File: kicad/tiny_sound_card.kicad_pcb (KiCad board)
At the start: 2 copper layers, 91 x 55 mm, 46 parts, among them CON1 BARREL_JACK, IC1 ATMEGA328P-A, J1 TRS_JACK, M1 DFR0299, P1 EXT_PWR, P10 M3Drill, P2 SPKOUT, P4 EXT_I2C, P4 M3Drill, P5 EXT_SW0, P6 EXT_UART, P7 EXT_SPI/ISP, P8 M3Drill, P9 M3Drill, SW1 SlideSW, SW2 SW_PUSH, SW3 SW_PUSH, SW4 SW_PUSH, SW5 SlideSW, SW6 SW_PUSH, U1 STMPS2141S, Y1 16MHz

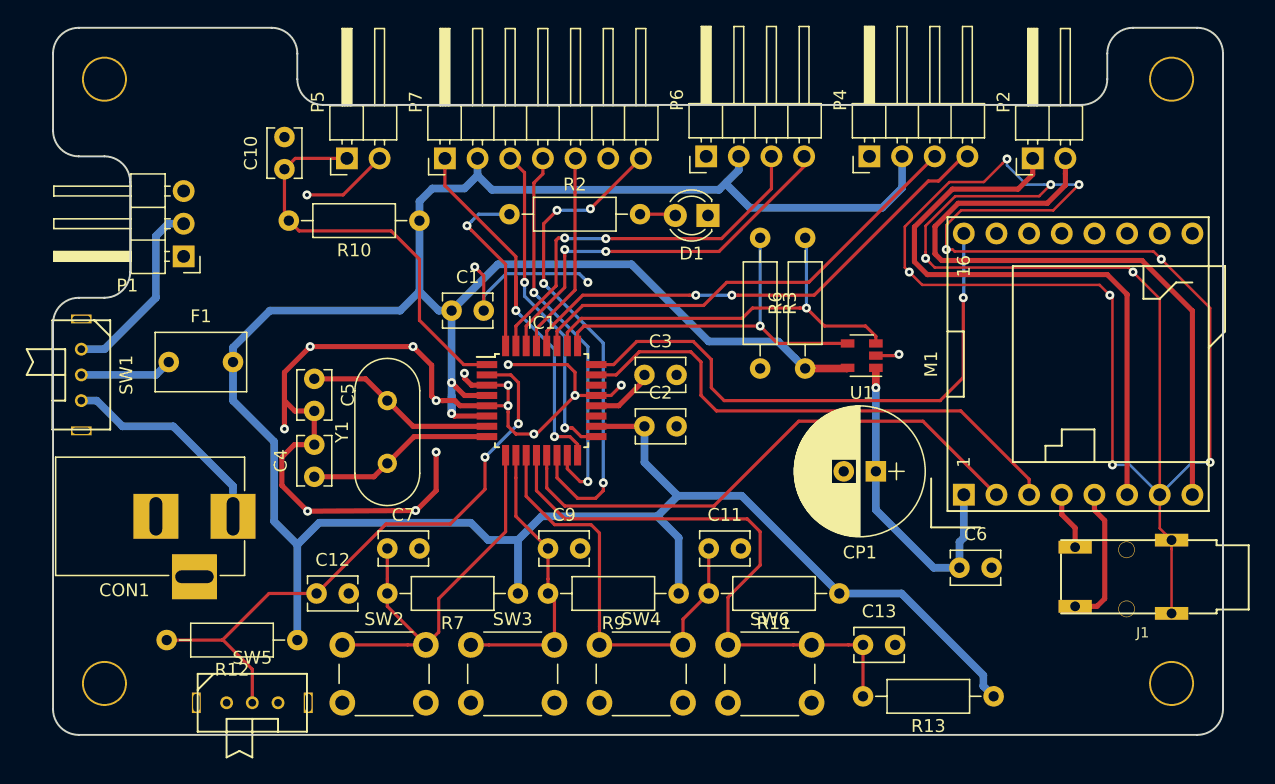
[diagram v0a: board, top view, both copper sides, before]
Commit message: ベタ配線
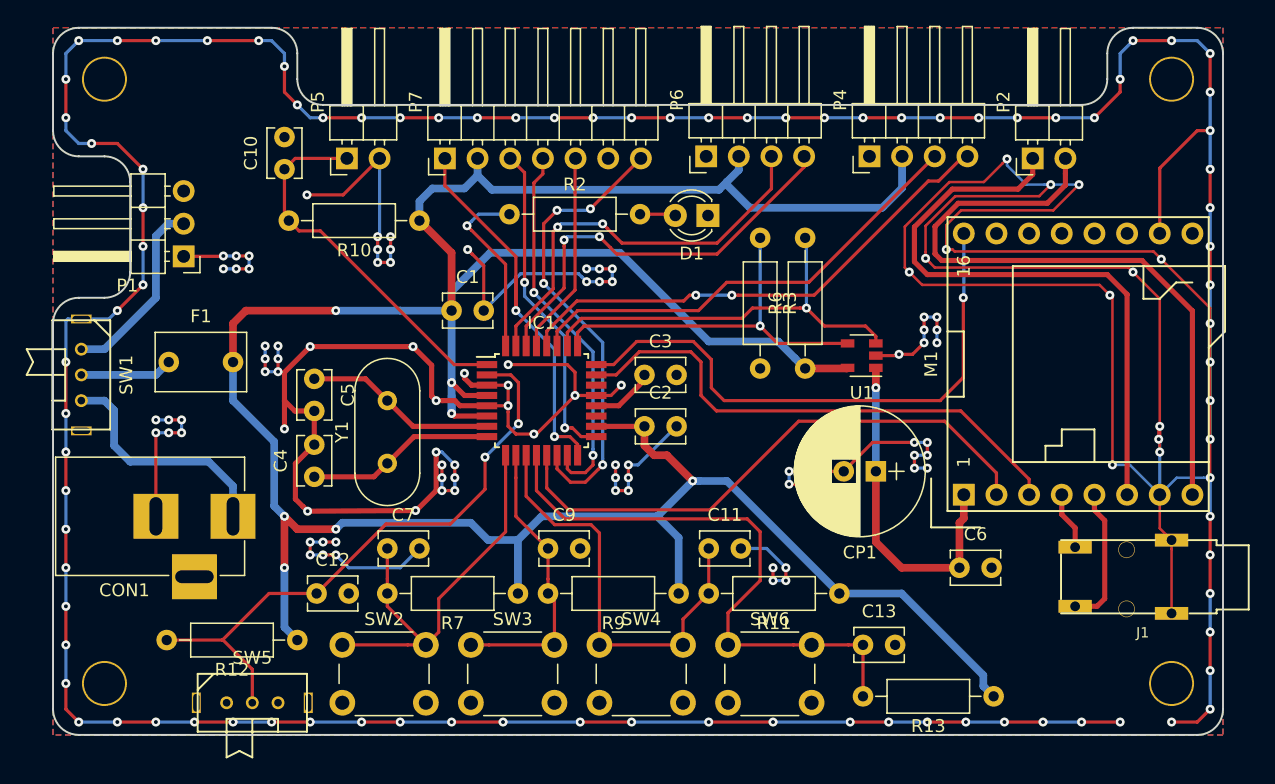
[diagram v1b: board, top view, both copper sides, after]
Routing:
- net GND: track 266.2 -> 674.7 mm, vias 29 -> 190
- net VCC: track 234.0 -> 239.8 mm, vias 2 -> 7
- net /D3: track 32.2 -> 29.4 mm
- net /D10: track 38.6 -> 35.9 mm
- net /D1: track 30.5 -> 32.2 mm
- net /CONN_VCC: track 16.9 -> 18.5 mm
- net /DFR_VCC: track 25.2 -> 26.7 mm
- net /ATMEGA_TX: track 43.2 -> 44.5 mm
- net /D0: track 31.2 -> 32.4 mm
- net /D11: track 30.2 -> 29.5 mm
- added copper zone on B.Cu, net GND
- added copper zone on F.Cu, net GND
